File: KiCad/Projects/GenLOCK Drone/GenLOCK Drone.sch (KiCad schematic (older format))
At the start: 0 parts

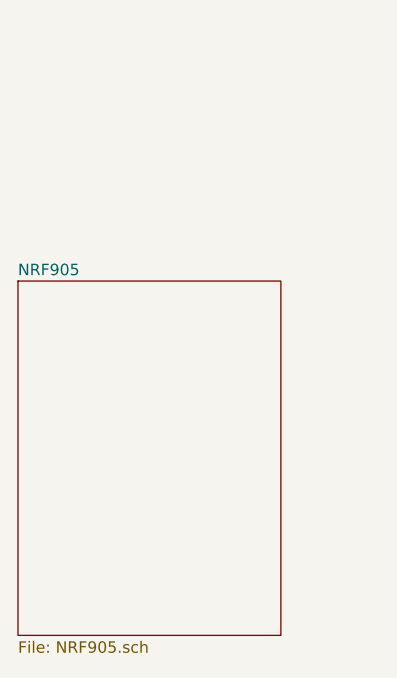
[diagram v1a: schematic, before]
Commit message: .
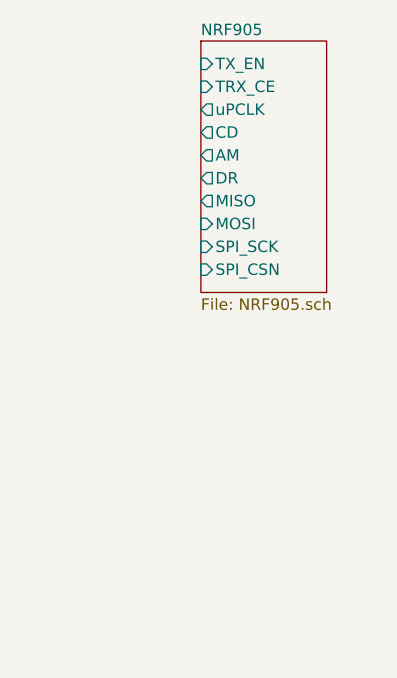
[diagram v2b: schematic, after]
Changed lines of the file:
@@
 encoding utf-8
 Sheet 1 2
-Title ""
-Date ""
-Rev ""
+Title "Drone PCB Schematic"
+Date "2019-05-28"
+Rev "1"
 Comp ""
 Comment1 ""
 Comment2 ""
-Comment3 ""
-Comment4 ""
+Comment3 "By Nathan Pendergrast"
+Comment4 "Gen:LOCK Drone Project"
 $EndDescr
 $Sheet
-S 9300 1900 1150 1550
+S 10100 850  550  1100
 U 5CECA62C
 F0 "NRF905" 50
 F1 "NRF905.sch" 50
+F2 "TX_EN" I L 10100 950 50
+F3 "TRX_CE" I L 10100 1050 50
+F4 "uPCLK" O L 10100 1150 50
+F5 "CD" O L 10100 1250 50
+F6 "AM" O L 10100 1350 50
+F7 "DR" O L 10100 1450 50
+F8 "MISO" O L 10100 1550 50
+F9 "MOSI" I L 10100 1650 50
+F10 "SPI_SCK" I L 10100 1750 50
+F11 "SPI_CSN" I L 10100 1850 50
 $EndSheet
 $EndSCHEMATC
